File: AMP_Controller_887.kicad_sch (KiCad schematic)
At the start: 65 parts, among them J1 Conn_PIC_ICSP_ICD, J3 4P_I2C, J4 Conn_01x13_Socket, J5 Conn_01x13_Socket, J6 2P_POWER, J7 USB_Mini_B_90_Angled, SW1 SW_RST, SW2 SW_PR21, X1 16MHz

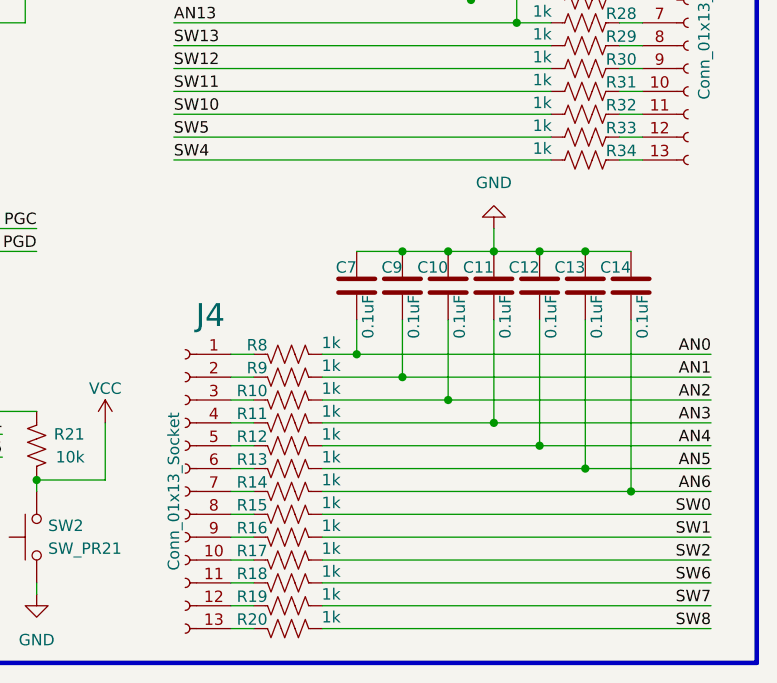
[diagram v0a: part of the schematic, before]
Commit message: Finished layout.
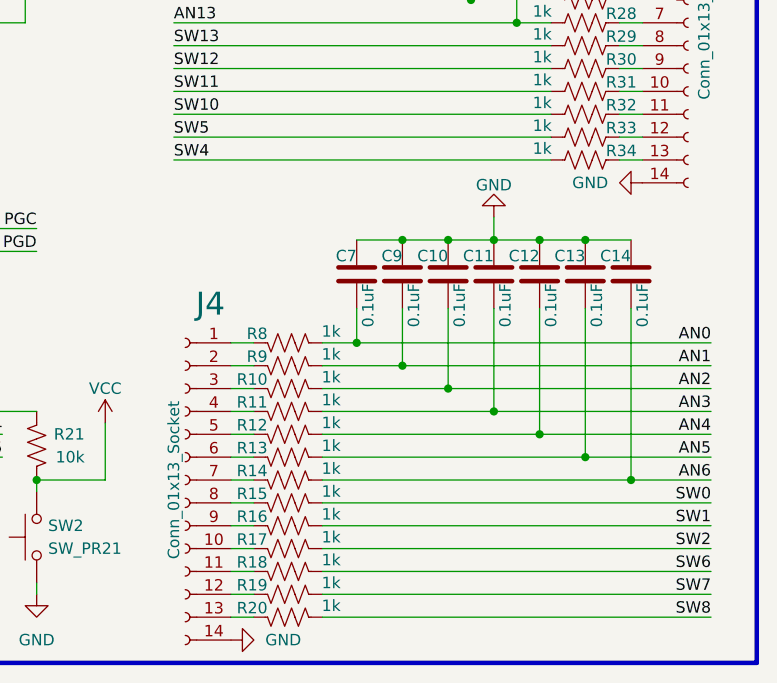
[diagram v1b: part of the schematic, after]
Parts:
- J4, J5: footprint Connector_PinSocket_2.54mm:PinSocket_1x13_P2.54mm_Vertical -> Connector_PinSocket_2.54mm:PinSocket_1x14_P2.54mm_Vertical; symbol Connector:Conn_01x13_Socket -> Connector:Conn_01x14_Socket
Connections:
- net GND: now also J4.14 (Pin_14), J5.14 (Pin_14)
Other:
- moved on the sheet: C10, C11, C12, C13, C14, C7, C9, R10, R11, R12, R13, R14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
